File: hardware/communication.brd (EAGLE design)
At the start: 33.5 x 34.6 mm, 44 parts, among them J1 MICRO_USB_B_HIROSE_ZX62-B-5PA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, SW1 TVAF06-A020B-R, U2 NJM12888F, X1 FA-238

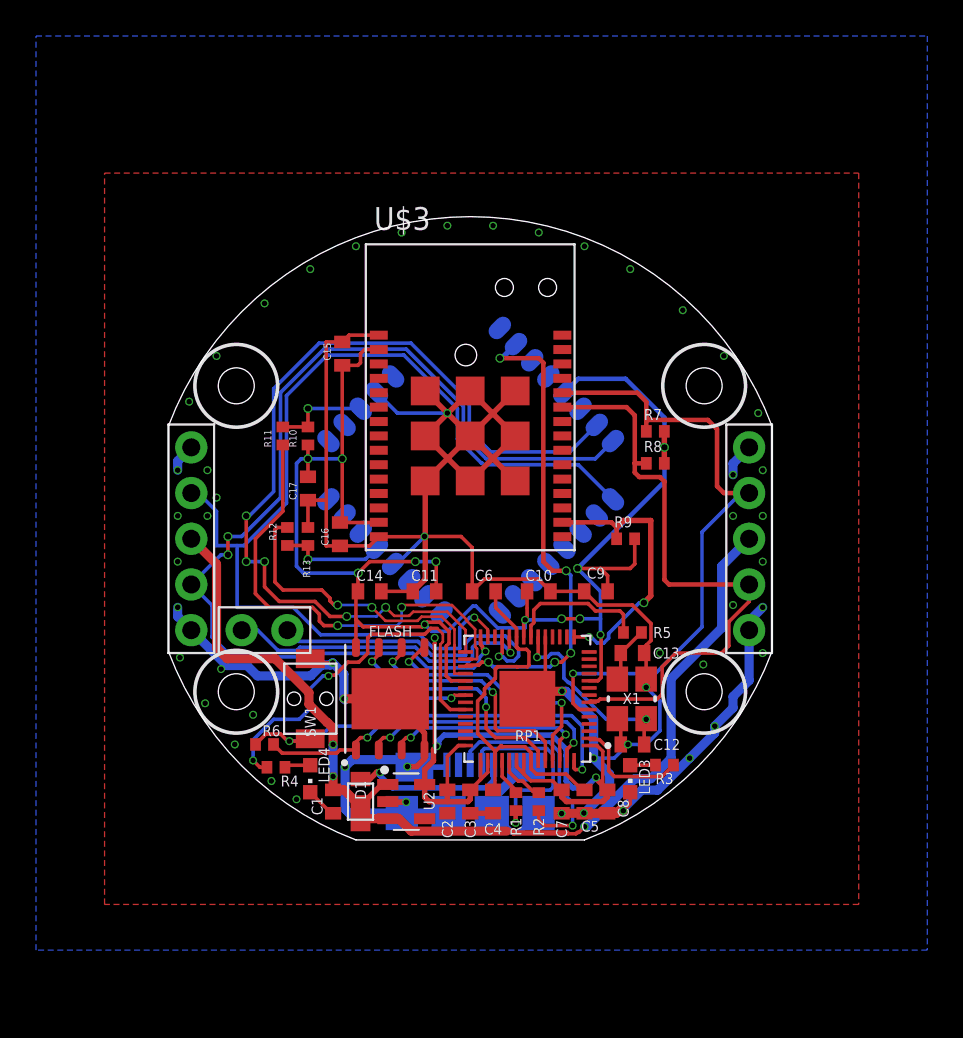
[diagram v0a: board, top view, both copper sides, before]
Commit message: Revert "communicationの層が一応完成しました。確認お願いします"
This reverts commit c7c23561daafb7c0ad8373af90d18b3355d51587.
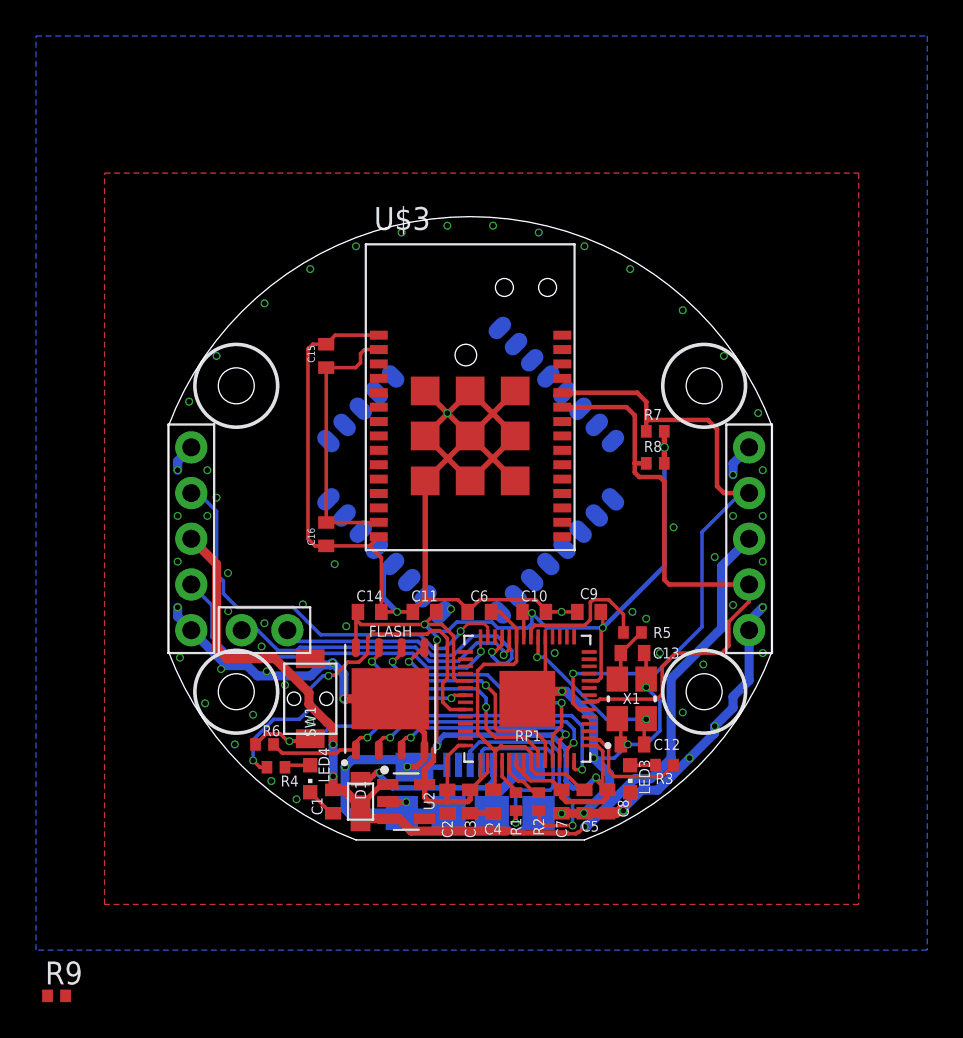
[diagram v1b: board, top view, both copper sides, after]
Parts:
- removed C17: 0.1µ, rcl:C0402
- removed R10, R13: 10k, rcl:R0402
- removed R11, R12: 1k, rcl:R0402
- moved R9 40.6 mm to (-23.0, -25.4)
- moved C9 1.20 mm to (6.60, -4.06)
- moved C10 1.17 mm to (3.56, -4.06)
- moved C6 1.17 mm to (0.51, -4.06)
- moved C11 1.14 mm to (-2.54, -4.06)
- moved C14 1.14 mm to (-5.59, -4.06)
- moved C15 0.90 mm to (-8.00, 10.2)
- moved C16 0.76 mm to (-8.00, 0.25)
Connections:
- removed net CTS0: RP1.29, U$1.7
- removed net TWE_PGM: RP1.31, U$1.2
- removed net TWE_RESET: R12.1, R12.2, R13.1, RP1.32, U$1.21
- removed net TWE_SLEEP: R10.2, R11.1, R11.2, RP1.30, U$1.27
- new net SPI0_CS: RP1.32
- new net SPI0_MISO: RP1.31
- new net SPI0_MOSI: RP1.30
- new net SPI0_SCK: RP1.29
- new net SPI1_MISO: RP1.15
- new net SPI1_MOSI: RP1.18
- new net SPI1_SCK: RP1.17
- new net VCC: U$1.5
- net GND: no longer C17.1, R13.2
- net RX0: no longer U$1.8
- net TX0: no longer U$1.9
- net VDD: no longer C17.2, R10.1, U$1.5
- net WKUP: no longer RP1.15
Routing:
- net CTS0: track 49.8 -> 0.00 mm, vias 5 -> 0
- net RX0: track 57.7 -> 20.5 mm, vias 3 -> 1
- net VDD: track 137.3 -> 101.9 mm, vias 15 -> 7
- net TX0: track 58.3 -> 23.7 mm
- net TWE_SLEEP: track 31.3 -> 0.00 mm, vias 3 -> 0
- net TWE_PGM: track 27.2 -> 0.00 mm, vias 5 -> 0
- net TWE_RESET: track 24.1 -> 0.00 mm, vias 3 -> 0
- net WKUP: track 15.7 -> 0.00 mm, vias 2 -> 0
- net GND: track 185.5 -> 174.2 mm, vias 54 -> 71
- net 1V2: track 21.4 -> 19.7 mm
- net XIN1: track 10.9 -> 10.2 mm
